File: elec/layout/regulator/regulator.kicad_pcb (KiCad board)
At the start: 2 copper layers, 13 parts, among them U1 _Texas_Instruments_TPS56637RP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

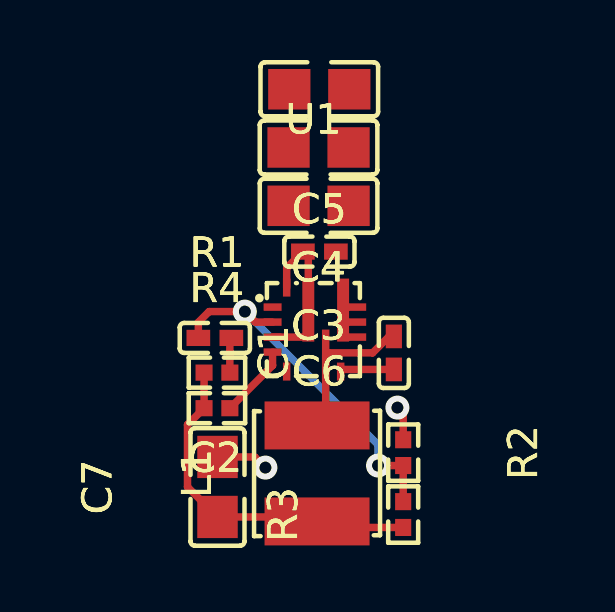
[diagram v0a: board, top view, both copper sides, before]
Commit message: Build full
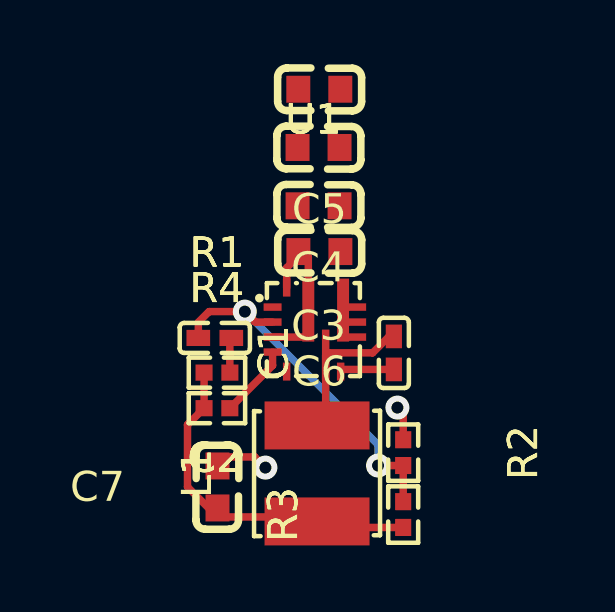
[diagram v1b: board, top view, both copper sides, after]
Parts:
- C3, C4, C5: value 4.7µF ±10% 25V X5R -> 100nF ±10% 50V X7R; footprint lcsc:C0805 -> lcsc:C0603
- C6: value 100nF ±10% 16V X7R -> 100nF ±10% 50V X7R; footprint lcsc:C0402 -> lcsc:C0603
- C7: value 47µF ±20% 6.3V X5R -> 100nF ±10% 50V X7R; footprint lcsc:C0805 -> lcsc:C0603
- L1: value 3.3µH ±20% 4A 73mΩ -> 3.3µH ±20% infHz 4A 73mΩ
- R1: value 22kΩ ±1% 62.5mW -> 20kΩ ±1% 62.5mW
- R2: value 8.2kΩ ±1% 62.5mW -> 10kΩ ±1% 62.5mW
- R3: value 68kΩ ±1% 62.5mW -> 75kΩ ±1% 62.5mW
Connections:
- C1 pad 2: net-6 -> net-5
- C2 pad 1: net-4 -> net
- C2 pad 2: net-5 -> net-1
- C3 pad 1: net -> net-2
- C3 pad 2: net-1 -> net-3
- C4 pad 1: net -> net-2
- C4 pad 2: net-1 -> net-3
- C5 pad 1: net -> net-2
- C5 pad 2: net-1 -> net-3
- C6 pad 1: net -> net-2
- C6 pad 2: net-1 -> net-3
- C7 pad 1: net-2 -> net-4
- C7 pad 2: net-1 -> net-3
- L1 pad 1: net-2 -> net-4
- L1 pad 2: net-6 -> net-5
- R1 pad 1: net-2 -> net-4
- R1 pad 2: net-4 -> net
- R2 pad 1: net-1 -> net-3
- R2 pad 2: net-5 -> net-1
- R3 pad 1: net-2 -> net-4
- R3 pad 2: net-5 -> net-1
- R4 pad 1: net-2 -> net-4
- R4 pad 2: net-3 -> net-6
- U1 pad 10: net-1 -> net-3
- U1 pad 2: net-5 -> net-1
- U1 pad 3: net-1 -> net-3
- U1 pad 4: net-3 -> net-6
- U1 pad 6: net-6 -> net-5
- U1 pad 8: net -> net-2
- U1 pad 9: net-1 -> net-3
